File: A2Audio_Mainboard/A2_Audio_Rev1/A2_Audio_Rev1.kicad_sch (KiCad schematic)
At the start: 34 parts, among them J2 AudioJack3, J3 BOOT_JUMPER, J7 SJ2-35954B-SMT-TR, SW1 SW_Push, SW2 WIFI_SLIDER, SW3 RotaryEncoder_Switch, SW4 BT_SLIDER, SW5 SW_PREV, SW6 SW_NEXT, SW7 SW_PLAY, U15 CM5108000, U23 LTC2954ITS8-1_TRPBF

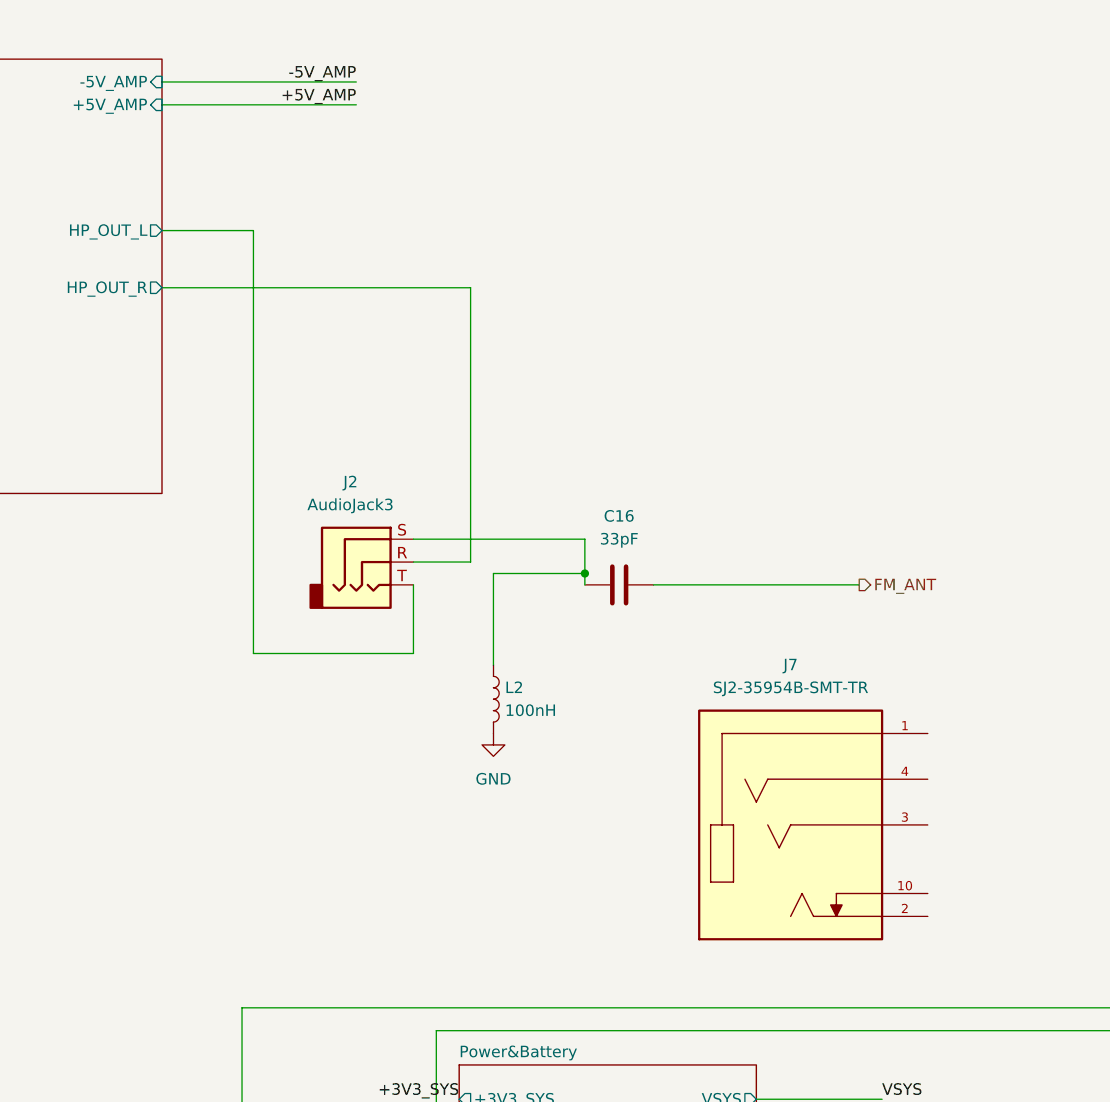
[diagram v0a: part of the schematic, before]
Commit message: More Refinement
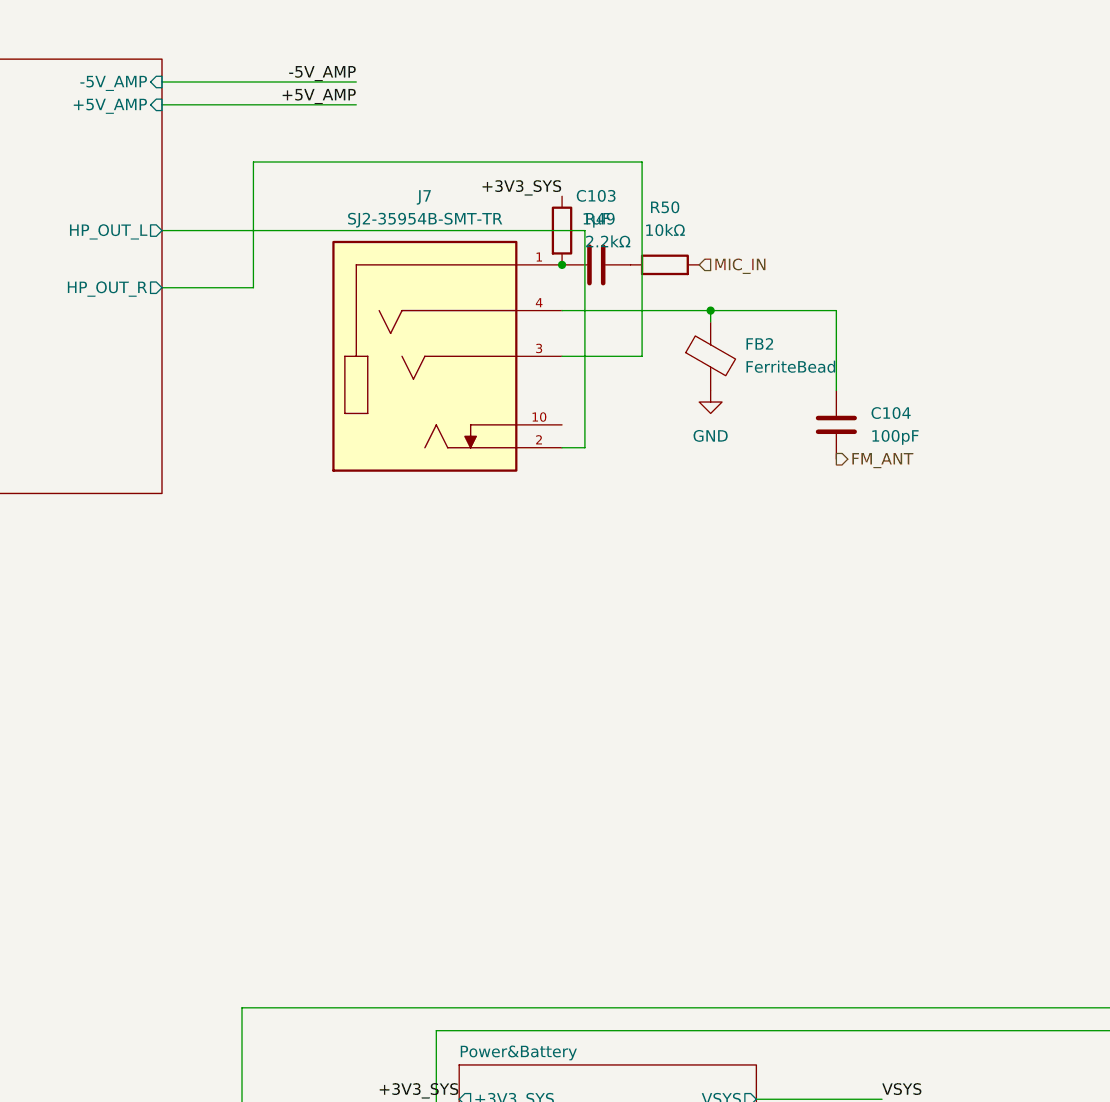
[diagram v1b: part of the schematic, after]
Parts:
- removed C16: 33pF, Capacitor_SMD:C_0402_1005Metric, symbol symbols:C
- removed J2: AudioJack3, symbol symbols:AudioJack3
- removed L2: 100nH, symbol symbols:L
- added C103: 1µF, symbol symbols:C
- added C104: 100pF, symbol symbols:C
- added FB2: FerriteBead, symbol symbols:FerriteBead
- added R49: 2.2kΩ, symbol symbols:R
- added R50: 10kΩ, symbol symbols:R
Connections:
- net +3V3_SYS: now also R49.1
- net Audio_Engine/HP_OUT_L: now also J7.2
- net Audio_Engine/HP_OUT_R: now also J7.3
- net FM_ANT: now also C104.2
- net GND: now also FB2.2
- net at J7.1: now also C103.1, R49.2
- net at J7.4: now also C104.1, FB2.1
- new net: C103.2, R50.1
- new net MIC_IN: R50.2
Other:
- moved on the sheet: J7
